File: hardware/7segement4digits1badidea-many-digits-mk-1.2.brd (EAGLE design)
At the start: 41 x 16 mm, 8 parts

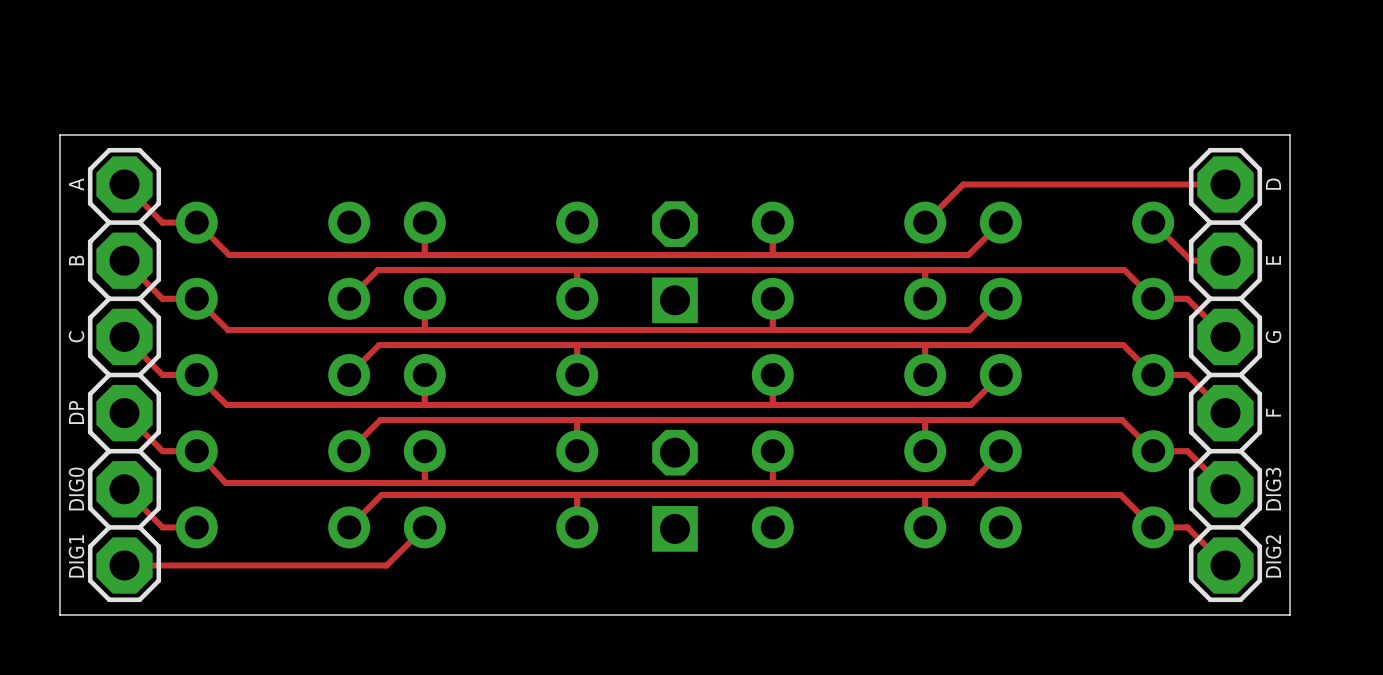
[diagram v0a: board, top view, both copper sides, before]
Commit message: lots of terribad ideas here
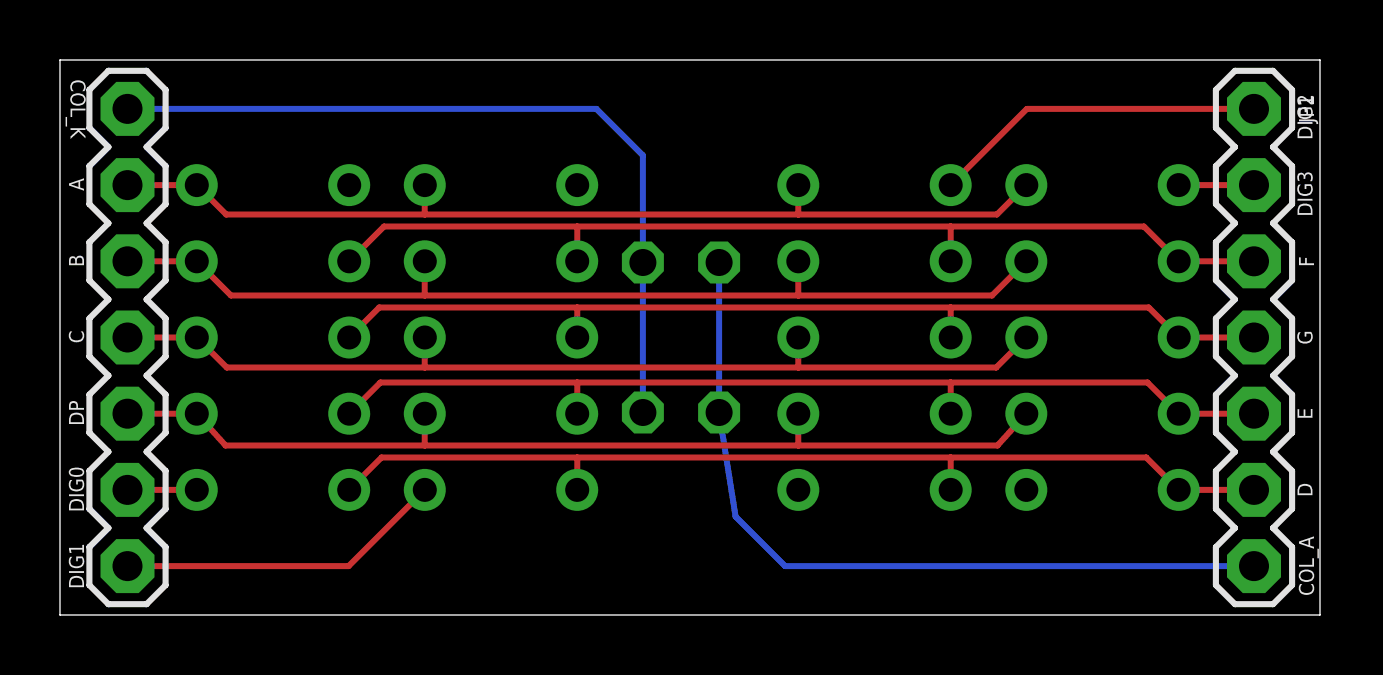
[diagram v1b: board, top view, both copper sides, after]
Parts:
- removed JP2: M06-NOBS-PTH, A_butts:1X06_NOLOCK_FUCKITALL
- added JP3: (no value), A_butts:1X07
- JP1: value M06-NOBS-PTH -> (none); device A_butts:1X06_NOLOCK_FUCKITALL -> A_butts:1X07
- LED1, LED2: value LED3MM -> LED3MM-LESS; device A_butts:LED3MM -> A_butts:LED3MM-LESSSILK
- moved JP1 40.6 mm to (39.8, 16.9), turned to 270 degrees
- moved LED2 2.62 mm to (20.7, 6.75), turned to 0 degrees
- moved DIGIT3 1.51 mm to (34.8, 9.25)
- moved DIGIT2 1.51 mm to (27.1, 9.25)
- moved DIGIT0 1.25 mm to (7.10, 9.25)
- moved DIGIT1 1.25 mm to (14.7, 9.25)
- moved LED1 0.20 mm to (20.7, 11.8), turned to 0 degrees
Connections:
- new net N$2: JP3.7, LED1.K, LED2.K
- new net N$3: JP1.7, LED1.A, LED2.A
- net A: now also JP3.6; no longer JP1.6
- net B: now also JP3.5; no longer JP1.5
- net C: now also JP3.4; no longer JP1.4
- net D: now also JP1.6; no longer JP2.6
- net DIG0: now also JP3.2; no longer JP1.2
- net DIG1: now also JP3.1; no longer JP1.1
- net DIG2: now also JP1.1; no longer JP2.1
- net DIG3: now also JP1.2; no longer JP2.2
- net DP: now also JP3.3; no longer JP1.3
- net E: now also JP1.5; no longer JP2.5
- net F: now also JP1.3; no longer JP2.3
- net G: now also JP1.4; no longer JP2.4
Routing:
- net N$3: track 0.00 -> 26.5 mm
- net N$2: track 0.00 -> 26.4 mm
- net F: track 32.5 -> 33.4 mm
- net DIG0: track 2.94 -> 2.31 mm
- net DIG2: track 10.5 -> 11.2 mm
- net B: track 32.7 -> 33.2 mm
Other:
- board size 41 x 16 mm -> 42 x 18.5 mm
- board text added: "COL_A"
- board text added: "COL_K"
